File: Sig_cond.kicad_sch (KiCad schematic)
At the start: 68 parts, among them U401 TSV912IDT, U403 TSV912IDT

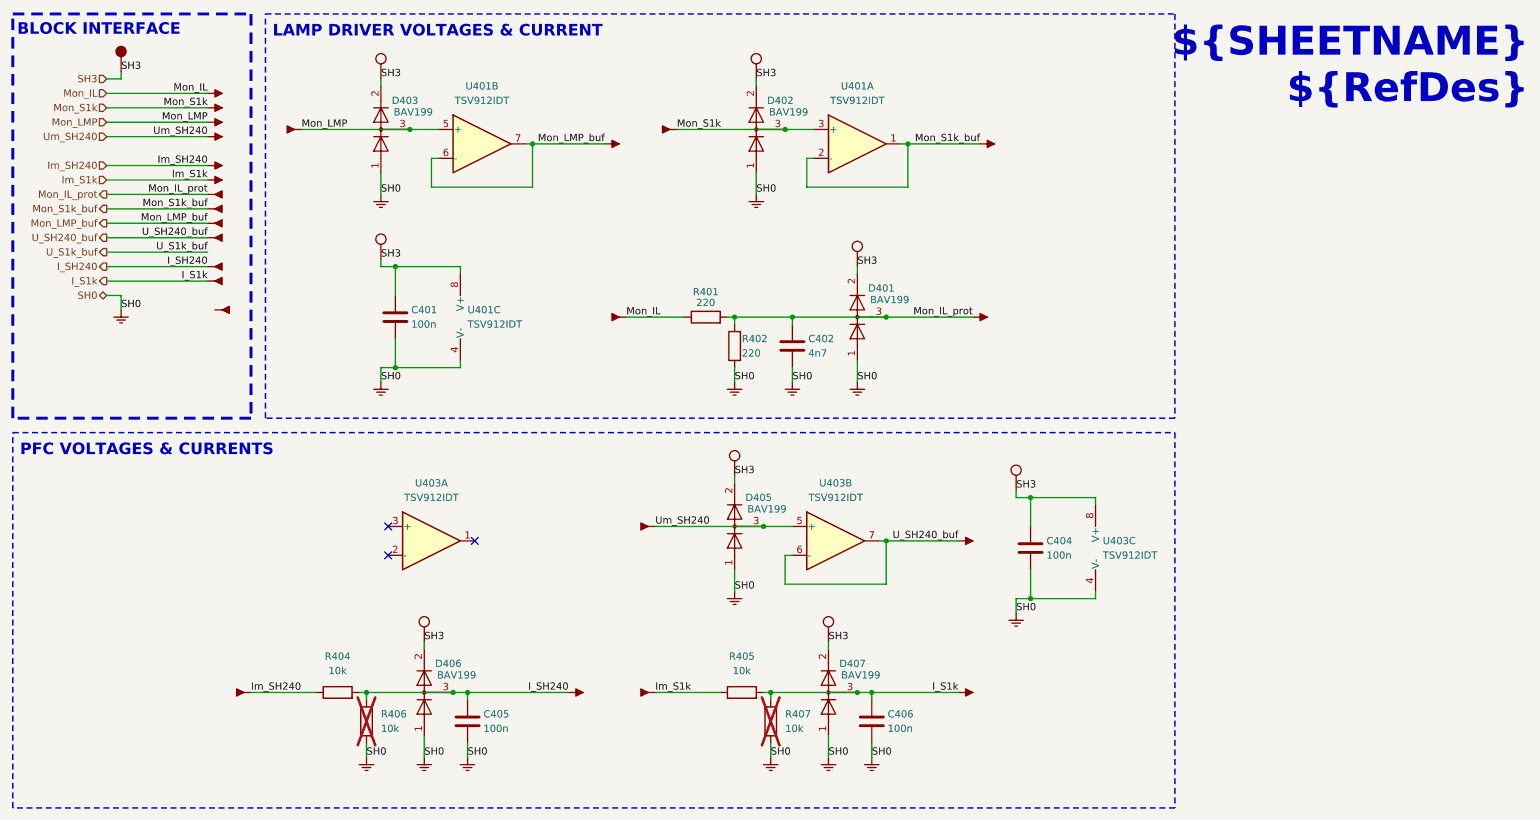
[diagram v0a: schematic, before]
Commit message: Sch update in progres
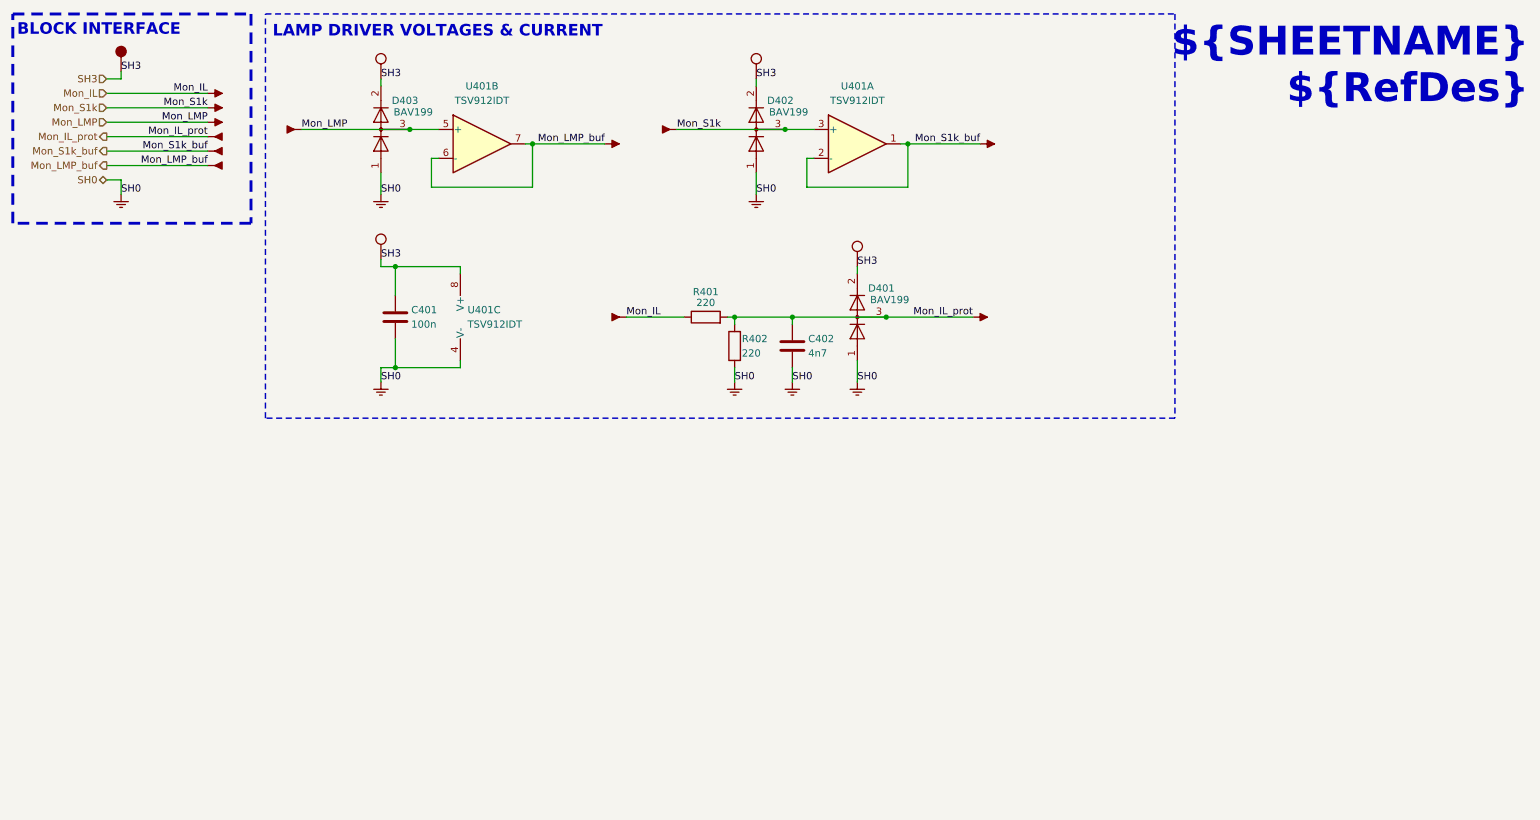
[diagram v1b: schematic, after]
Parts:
- removed C404, C405, C406: 100n, Capacitor_SMD:C_0603_1608Metric_Pad1.08x0.95mm_HandSolder, symbol Device:C
- removed D405, D406, D407: BAV199, Package_TO_SOT_SMD:SOT-23, symbol Diode:BAV99
- removed P306, P866, P867, P868, P875, P877, P878: ~, symbol personal:Cosmetic_IN
- removed P450, P452, P574, P599, P606, P608: ~, symbol personal:Cosmetic_OUT
- removed P593, P595, P603, P604: ~, symbol personal:Cosmetic_PWR
- removed P824, P825, P826, P827, P828, P829, P830, P831: ~, symbol personal:Cosmetic_GND
- removed R404, R405, R406, R407: 10k, Resistor_SMD:R_0603_1608Metric_Pad0.98x0.95mm_HandSolder, symbol Device:R
- removed U403: TSV912IDT, Package_SO:SOIC-8_3.9x4.9mm_P1.27mm, symbol Amplifier_Operational:TSV912IDT
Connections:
- no-connect marks 3 -> 0
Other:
- note removed: "PFC VOLTAGES & CURRENTS"
